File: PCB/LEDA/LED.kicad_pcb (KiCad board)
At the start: 2 copper layers, 70 x 70 mm, 25 parts, among them J1 USB_A, J2 Conn_01x03, J3 TC2030-USB-NL-DS, U1 ICS43434_MEMS_Mic, U2 ESP32-S3-MINI-1, U5 MD8942

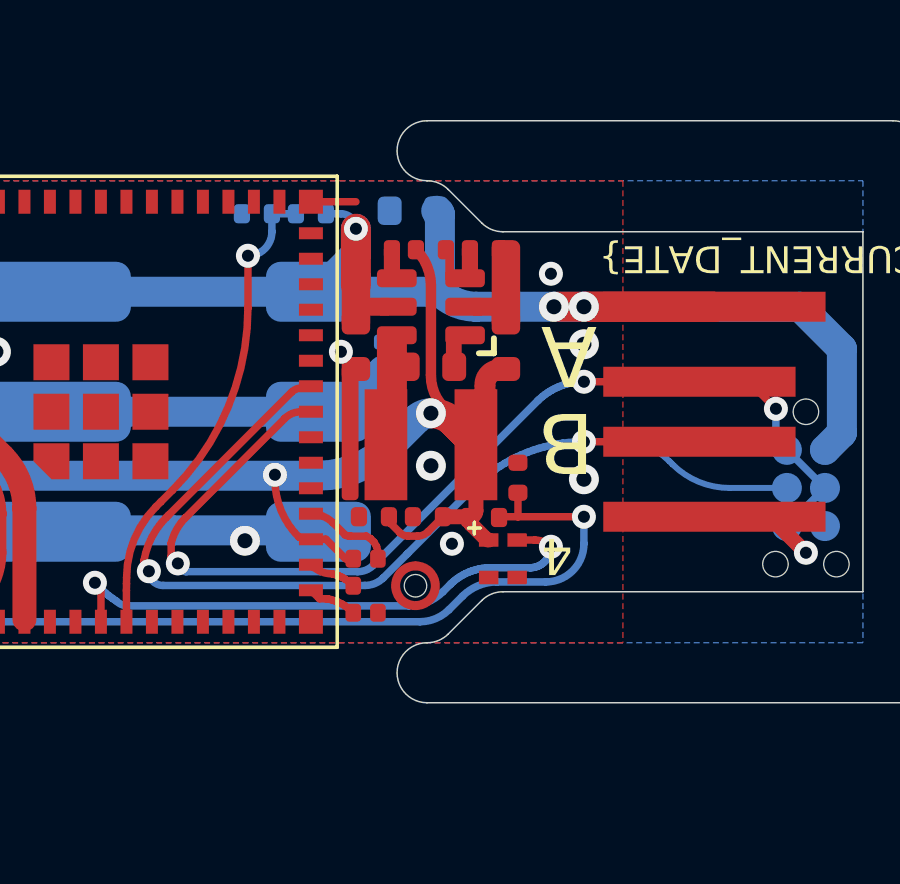
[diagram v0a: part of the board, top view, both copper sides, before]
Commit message: Not a good case, but started one, and some cleaner renders
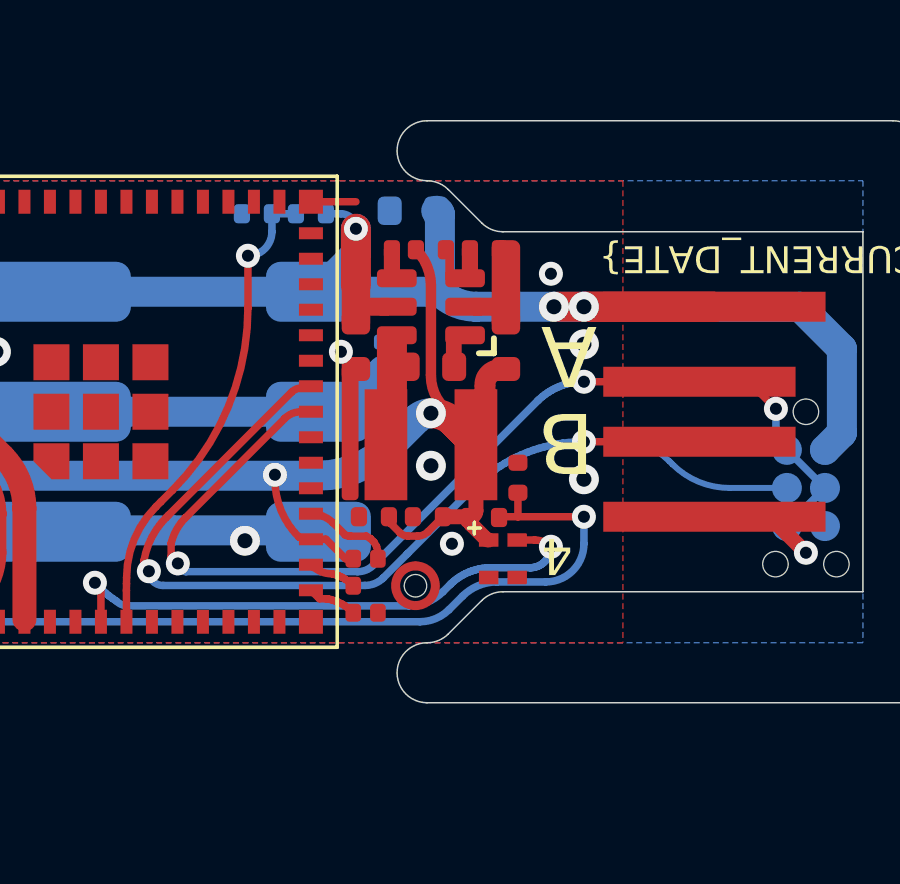
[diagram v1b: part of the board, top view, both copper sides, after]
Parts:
- J2: footprint RevK:WAGO-2060-453-998-404 -> RevK:WAGO-2060-453-998-404-O
